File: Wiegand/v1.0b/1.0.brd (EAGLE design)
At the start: 91.6 x 46.5 mm, 64 parts, among them CON1 SPI, IC1 REG1117, Q3 BSP75, Q5 BSP75, U1 MPL3115A2LGA8, X3 16MHz, X4 MINI-USB

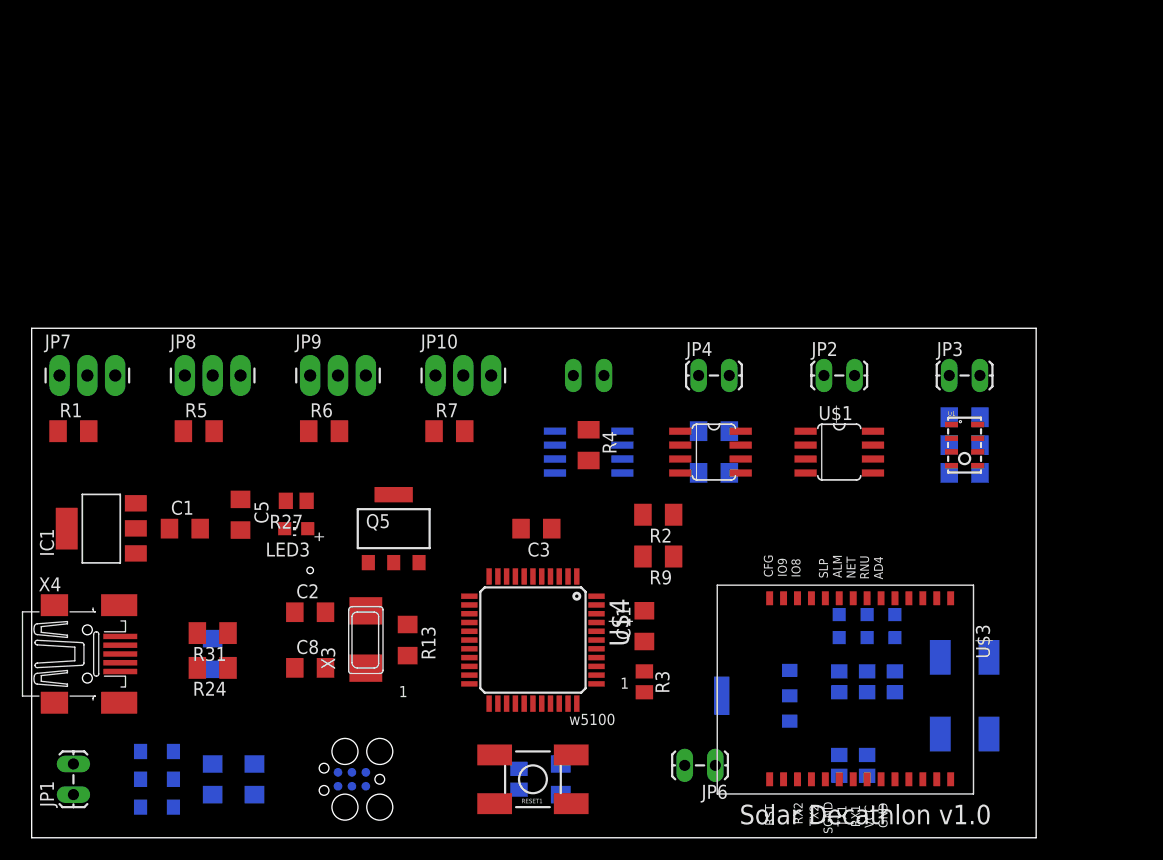
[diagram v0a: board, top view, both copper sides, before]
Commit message: Update wiegand
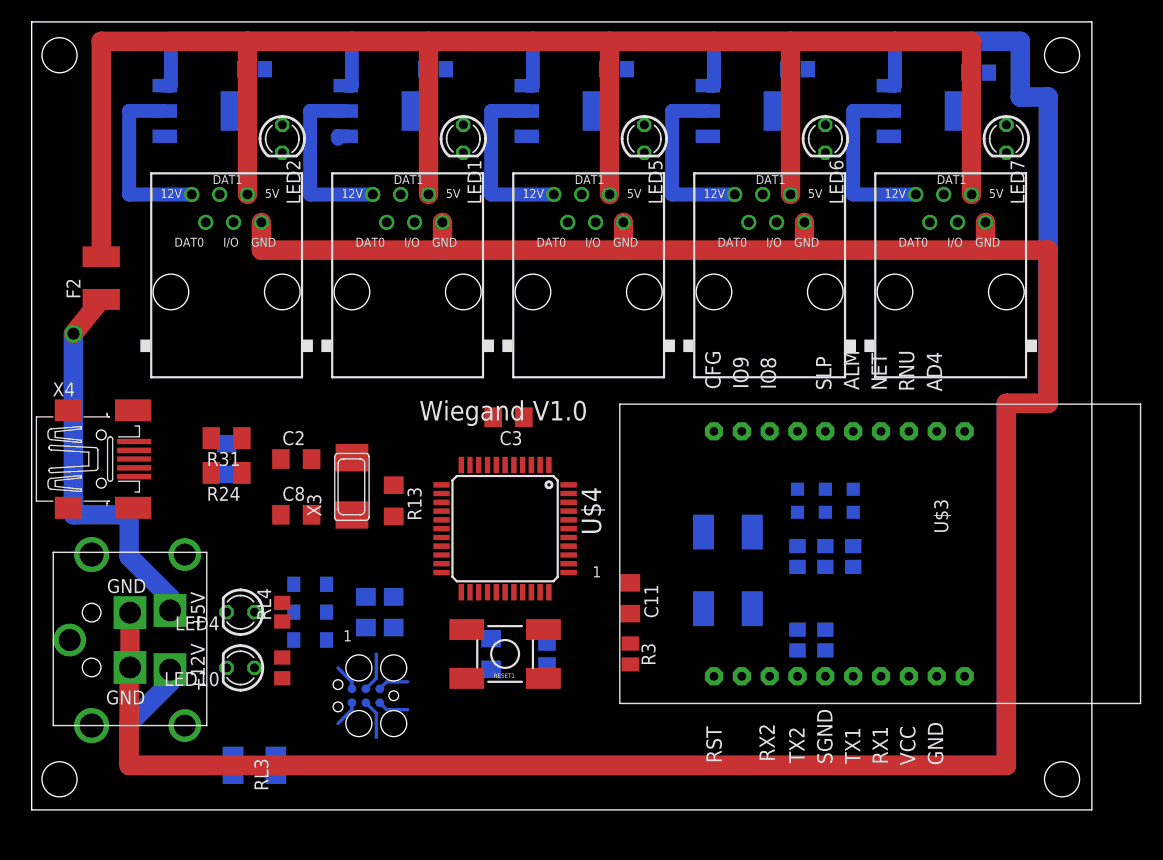
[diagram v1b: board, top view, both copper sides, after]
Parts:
- removed C1, C14, C5: 10uF, rcl:C1206
- removed C13, C15, C4: 100nF, rcl:C1206
- removed C6: 220nF, rcl:C1206
- removed IC1: REG1117, burr-brown:SOT223
- removed JP1, JP2, JP3, JP4, JP5, JP6: (no value), SparkFun:1X02_LOCK_LONGPADS
- removed JP10, JP7, JP8, JP9: (no value), SparkFun:1X03_LONGPADS
- removed LED3: RED, adafruit:CHIP-LED0805
- removed R27: 1K, rcl:R0805
- removed R6, R7: 4.7k, resistor:M1206
- removed R9: 10k, resistor:M1206
- removed U$1: M24512, lpatiny:SO8
- removed U$2: CHIPCAP, lpatiny:CHIPCAP
- removed U$5: DS18B20, lpatiny:SO8
- removed U1: MPL3115A2LGA8, SparkFun-Sensors:LGA8
- added F1, F2: 0.5A, lpatiny:C1812
- added J1, J2, J3, J4, J5: RJ12, lpatiny:RJ12-STRAIGHT-WIEGAND
- added LED1, LED2, LED5, LED6, LED7: Blue, lpatiny:LED3MM
- added LED10, LED4: RED, lpatiny:LED3MM
- added Q1, Q2, Q4: BSP75, zetex:SOT223
- added R25: 10k, rcl:R0805
- added RL3: 1K, rcl:R0805
- added RL4: 1K, resistor:R0805
- added U$6: KPJX-4S-S, lpatiny:KPJX-4S-S
- Q3, Q5: device infineon:PG-SOT-223 -> zetex:SOT223
- R1, R4, R5: value 4.7k -> 10k; device resistor:M1206 -> rcl:R0805
- R2: device resistor:M1206 -> rcl:R0805
- U$3: value SZ05-ZIGBEESMD -> SZ05-ZIGBEE; device lpatiny:SZ05-ZIGBEE3 -> lpatiny:SZ05-ZIGBEE
- moved R5 78.3 mm to (86.4, 67.0), flipped to the bottom
- moved Q5 61.5 mm to (81.3, 63.5), flipped to the bottom, turned to 90 degrees
- moved Q3 56.2 mm to (48.3, 63.5), turned to 90 degrees
- moved R1 46.7 mm to (36.8, 67.3), flipped to the bottom
- moved R2 40.8 mm to (53.3, 67.3), flipped to the bottom, turned to 0 degrees
- moved R4 39.2 mm to (69.8, 67.3), flipped to the bottom, turned to 0 degrees
- moved CFG 24.4 mm to (63.5, 21.6)
- moved D2 22.6 mm to (25.4, 20.3)
- moved C10 20.7 mm to (30.5, 17.8)
- moved D3 20.7 mm to (25.4, 15.2)
- moved C12 19.8 mm to (33.0, 17.8)
- moved D4 18.9 mm to (25.4, 17.8)
- moved C7 17.8 mm to (17.8, 31.8)
- moved R24 17.8 mm to (17.8, 30.5)
- moved R31 17.8 mm to (17.8, 33.7)
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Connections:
- removed net $1: C13.2, C14.2, C15.2, JP3.1, U1.3
- removed net $12: JP2.1, U$1.4
- removed net $2: C4.2, JP4.1, U$2.2
- removed net $3: JP5.1, U$5.5
- removed net 3.3V: C1.1, C13.1, C14.1, C6.1, IC1.2, JP10.1, JP7.1, JP8.1, JP9.1, R1.1, R2.2, R27.2, R4.1, R5.1, R6.1, R7.1, R9.1, U$1.8, U$2.3, U$5.3, U1.1, U1.4
- removed net CTRL_GND: C6.2
- removed net GND_CONTROLLED: JP2.2, JP3.2, JP4.2, JP5.2, Q3.2, Q5.3
- removed net N$13: C15.1, U1.2
- removed net N$2: JP6.2, Q5.2
- removed net N$20: LED3.A, R27.1
- removed net N$6: C4.1, U$2.1
- removed net N$8: JP6.1, U$3.GND
- removed net N$9: JP10.2, R7.2
- removed net SCL: R9.2, U$1.6, U$2.8, U$4.18, U1.8
- removed net SDA: R2.1, U$1.5, U$2.7, U$4.19, U1.7
- removed net VCC: C10.1, C12.2, C5.1, D2.C, D3.C, D4.C, IC1.3, R15.2, U$4.14, U$4.2, U$4.24, U$4.34, U$4.44
- new net +12V: F1.2, Q1.3, Q2.3, Q3.3, Q4.3, Q5.3, RL3.2
- new net +5V/1: C10.1, C12.2, D2.C, D3.C, D4.C, R15.2, RL4.1, U$4.14, U$4.2, U$4.24, U$4.34, U$4.44
- new net D2*: J1.DAT0, U$4.19
- new net D3*: J1.DAT1, U$4.18
- new net D4*: J2.DAT0
- new net N$12: LED4.A, RL4.2
- new net N$17: LED2.A, R25.1
- new net N$19: LED6.A, R4.1
- new net N$22: J4.+12V, Q4.2, Q4.4, R4.2
- new net N$23: J1.+12V, Q1.2, Q1.4, R25.2
- new net N$29: LED7.A, R5.1
- new net N$31: J5.+12V, Q5.2, Q5.4, R5.2
- new net N$38: F2.1, U$6.+5V
- new net N$39: F1.1, U$6.+12V
- new net N$75: LED10.A, RL3.1
- net +5V: now also F2.2, J1.+5V, J2.+5V, J3.+5V, J4.+5V, J5.+5V; no longer JP1.1
- net A0: now also J5.I/O
- net A1: now also J3.I/O
- net A2: now also J2.I/O
- net A3: now also J1.I/O, J4.I/O
- net D10*: now also J3.DAT0
- net D11*: now also Q5.1
- net D12*: now also J3.DAT1
- net D13*: now also J4.DAT0
- net D5*: now also Q4.1
- net D6*: now also Q1.1
- net D7*: now also J2.DAT1
- net D8*: now also Q2.1
- net D9*: no longer Q5.1
- net GND: now also J1.GND, J2.GND, J3.GND, J4.GND, J5.GND, LED1.K, LED10.K, LED2.K, LED4.K, LED5.K, LED6.K, LED7.K, U$3.GND, U$3.SGND, U$6.GND1, U$6.GND2; no longer C1.2, C5.2, IC1.1, JP1.2, JP10.3, JP7.3, JP8.3, JP9.3, LED3.C, Q3.3, U$1.1, U$1.2, U$1.3, U$1.7, U$3.SND
- net GND1: now also U$3.RNU; no longer U$3.RUN
- net MISO: now also J4.DAT1
- net MOSI: now also J5.DAT1
- net N$1: now also LED1.A, R1.1; no longer R4.2, U$5.4
- net N$3: now also J2.+12V, Q2.2, Q2.4; no longer JP7.2
- net N$5: now also LED5.A, R2.1; no longer JP8.2, R5.2
- net N$7: now also J3.+12V, Q3.2, Q3.4, R2.2; no longer JP9.2, R6.2
- net SCK: now also J5.DAT0
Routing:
- net +12V: track 0.00 -> 239.5 mm
- net GND: track 0.00 -> 232.5 mm
- net +5V: track 0.00 -> 168.9 mm
- net N$38: track 0.00 -> 35.9 mm, vias 0 -> 1
- net N$39: track 0.00 -> 19.8 mm
- net N$7: track 0.00 -> 16.6 mm
- net N$3: track 0.00 -> 16.6 mm
- net N$23: track 0.00 -> 16.6 mm
- net N$22: track 0.00 -> 16.6 mm
- net N$31: track 0.00 -> 16.6 mm
- net SCK: track 0.00 -> 3.57 mm
- net MOSI: track 0.00 -> 3.57 mm
- net MISO: track 0.00 -> 2.80 mm
- net ISP+5V: track 0.00 -> 2.80 mm
- net RESET: track 0.00 -> 2.43 mm
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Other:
- board size 91.6 x 46.5 mm -> 96.7 x 71.9 mm
- board text added: "Wiegand V1.0"
- board text removed: "Solar Decathlon v1.0"
- board text removed: "w5100"
